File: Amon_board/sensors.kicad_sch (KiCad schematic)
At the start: 42 parts, among them J10 GTFP08131Y2HR, J11 Conn_01x03_Male, J12 Conn_01x06_Male, J13 Conn_01x04_Male, J14 Conn_01x04_Male, J15 Conn_01x06_Male, J6 Conn_02x04_Odd_Even, J7 Red leds, J8 White leds, J9 Conn_02x04_Odd_Even, M1 Servo_X+, M2 Servo_X-, M3 Servo_Y+, M4 Servo_Y-, Q1 BC817, Q2 BC817, U6 MPU-6050, U7 BME280

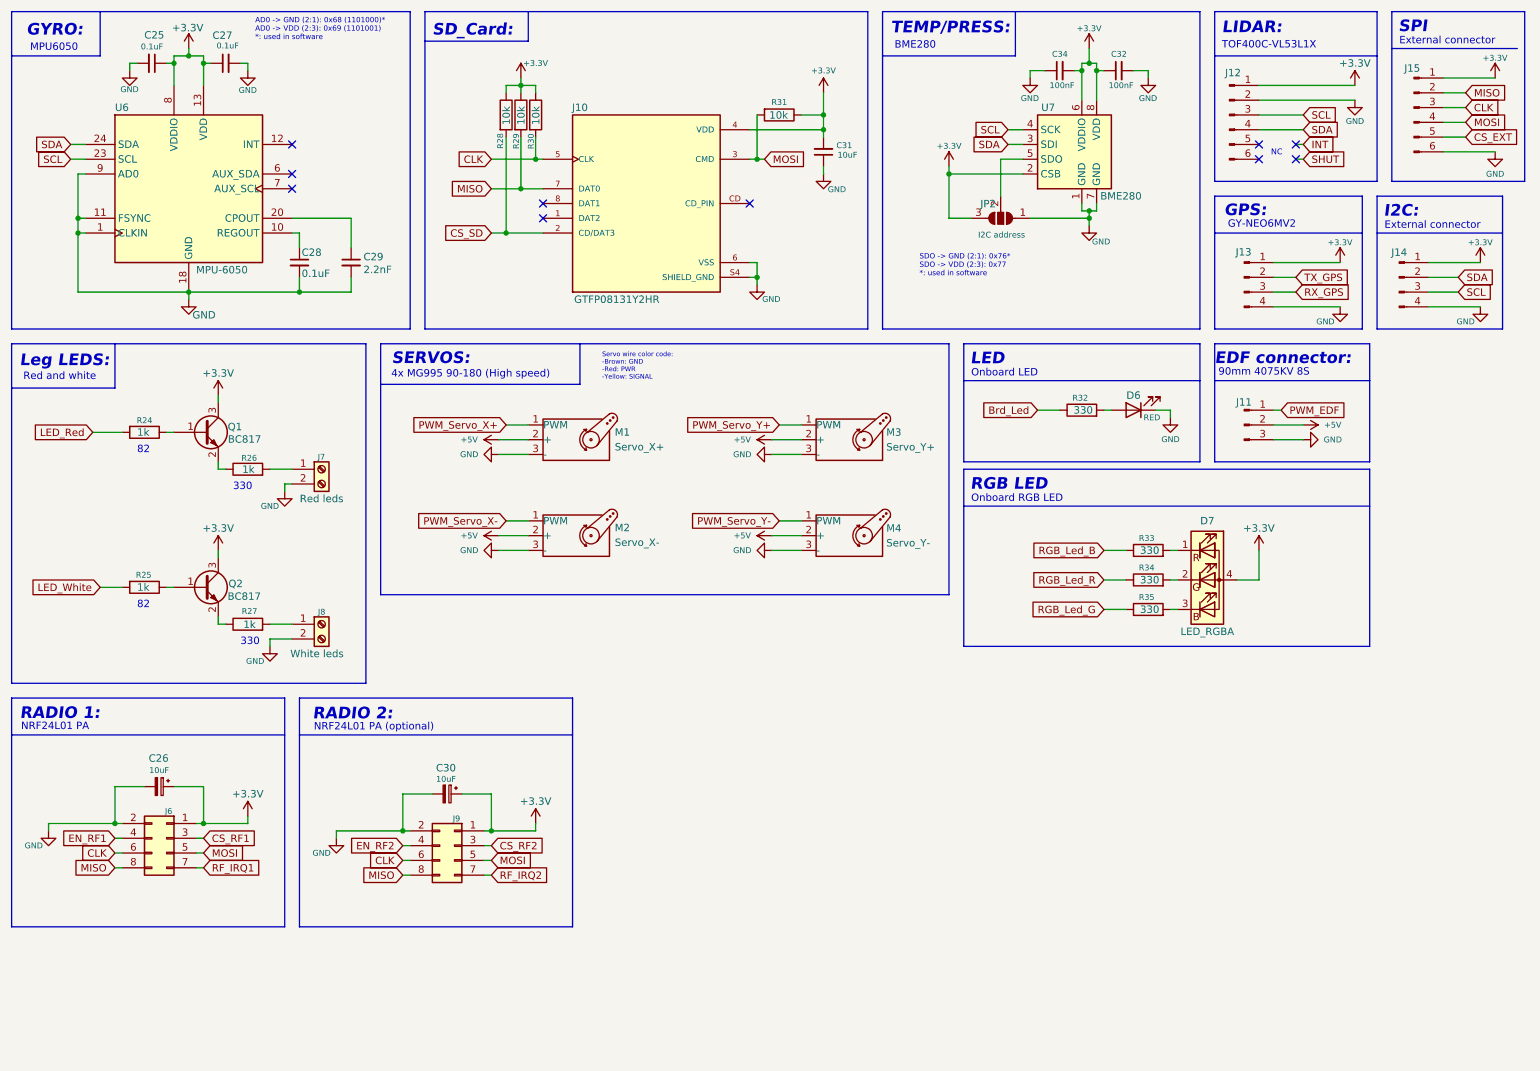
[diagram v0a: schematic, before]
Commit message: changed directories
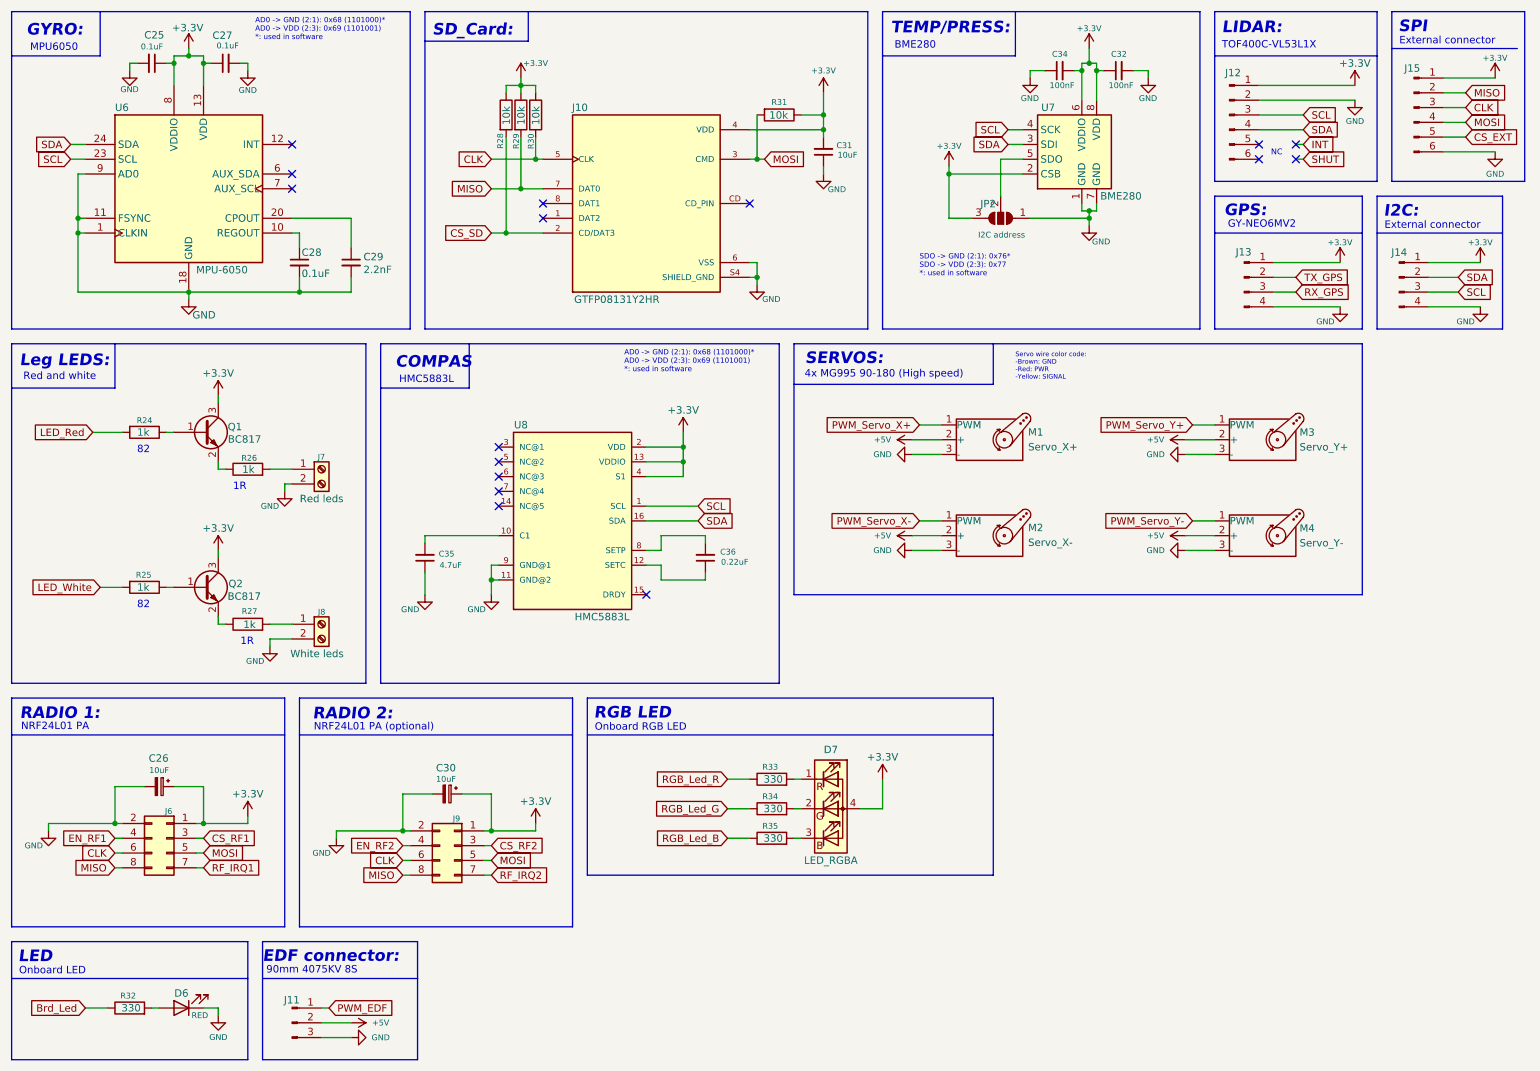
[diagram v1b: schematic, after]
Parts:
- added C35: 4.7uF, Capacitor_SMD:C_0603_1608Metric, symbol Device:C_Small
- added C36: 0.22uF, Capacitor_SMD:C_0603_1608Metric, symbol Device:C_Small
- added U8: HMC5883L, HMC5883L:LPCC-16, symbol HMC5883L:HMC5883L
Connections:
- net +3V3: now also U8.13 (VDDIO), U8.2 (VDD), U8.4 (S1)
- net GND: now also C35.1, U8.11 (GND@2), U8.9 (GND@1)
- net RGB_Led_B: now also R35.1; no longer R33.1
- net RGB_Led_G: now also R34.1; no longer R35.1
- net RGB_Led_R: now also R33.1; no longer R34.1
- net SCL: now also U8.1 (SCL)
- net SDA: now also U8.16 (SDA)
- new net: C35.2, U8.10 (C1)
- new net: C36.1, U8.12 (SETC)
- new net: C36.2, U8.8 (SETP)
- no-connect marks 10 -> 16
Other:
- note added: "1R"
- note added: "COMPAS"
- note added: "HMC5883L"
- note removed: "330"
- moved on the sheet: D6, D7, J11, M1, M2, M3, M4, R32, R33, R34, R35

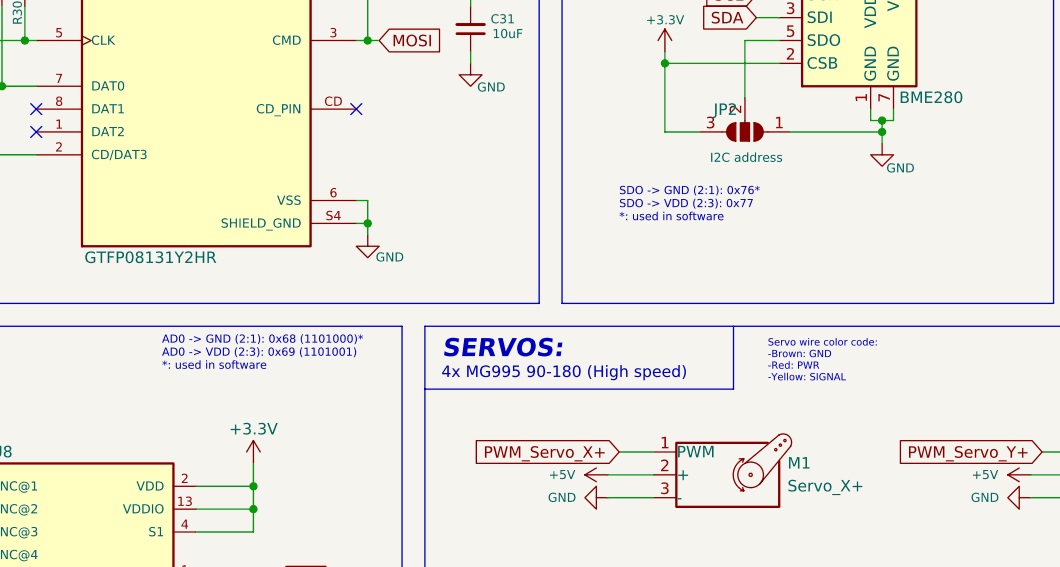
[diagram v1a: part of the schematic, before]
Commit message: added pictires
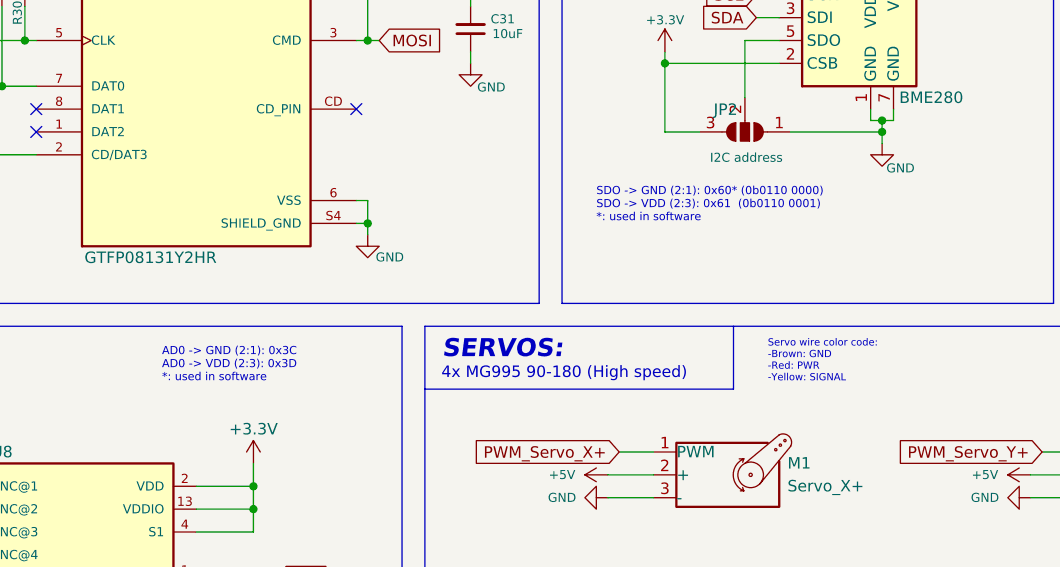
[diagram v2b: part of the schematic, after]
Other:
- note added: "AD0 -> GND (2:1): 0x3C AD0 -> VDD (2:3): 0x3D *: used in software"
- note added: "SDO -> GND (2:1): 0x60* (0b0110 0000) SDO -> VDD (2:3): 0x61 (0b0110 0001) *: used in software"
- note removed: "SDO -> GND (2:1): 0x76* SDO -> VDD (2:3): 0x77 *: used in software"
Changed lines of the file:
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@@
     (effects (font (size 1.27 1.27)) (justify left bottom))
   )
-  (text "AD0 -> GND (2:1): 0x68 (1101000)*\nAD0 -> VDD (2:3): 0x69 (1101001)\n*: used in software"
-    (at 120.65 77.47 0)
+  (text "AD0 -> GND (2:1): 0x3C\nAD0 -> VDD (2:3): 0x3D\n*: used in software"
+    (at 120.65 78.74 0)
     (effects (font (size 0.9 0.9)) (justify left bottom))
   )
@@
     (effects (font (size 2 2) (thickness 0.4) bold italic) (justify left bottom))
   )
-  (text "SDO -> GND (2:1): 0x76*\nSDO -> VDD (2:3): 0x77\n*: used in software"
-    (at 171.45 60.96 0)
+  (text "SDO -> GND (2:1): 0x60* (0b0110 0000)\nSDO -> VDD (2:3): 0x61  (0b0110 0001)\n*: used in software"
+    (at 168.91 60.96 0)
     (effects (font (size 0.9 0.9)) (justify left bottom))
   )
